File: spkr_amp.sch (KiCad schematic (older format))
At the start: 4 parts, among them U2 FSA2275UMX, U3 TPA2006D1DRBR

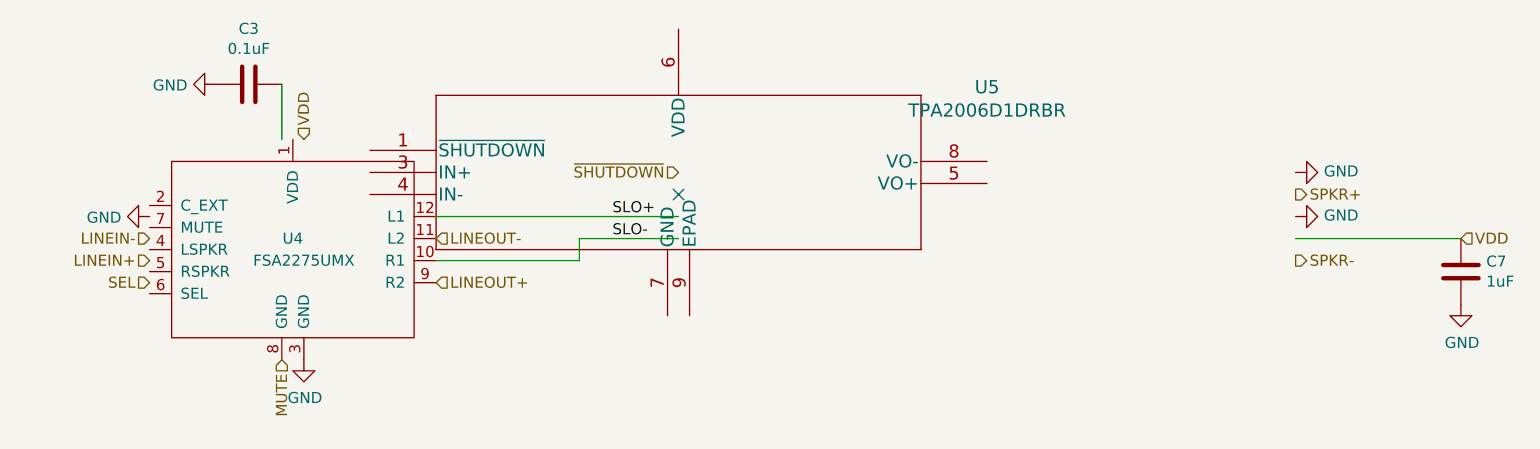
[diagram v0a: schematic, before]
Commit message: Lots of schematic cleanup and board tweaking
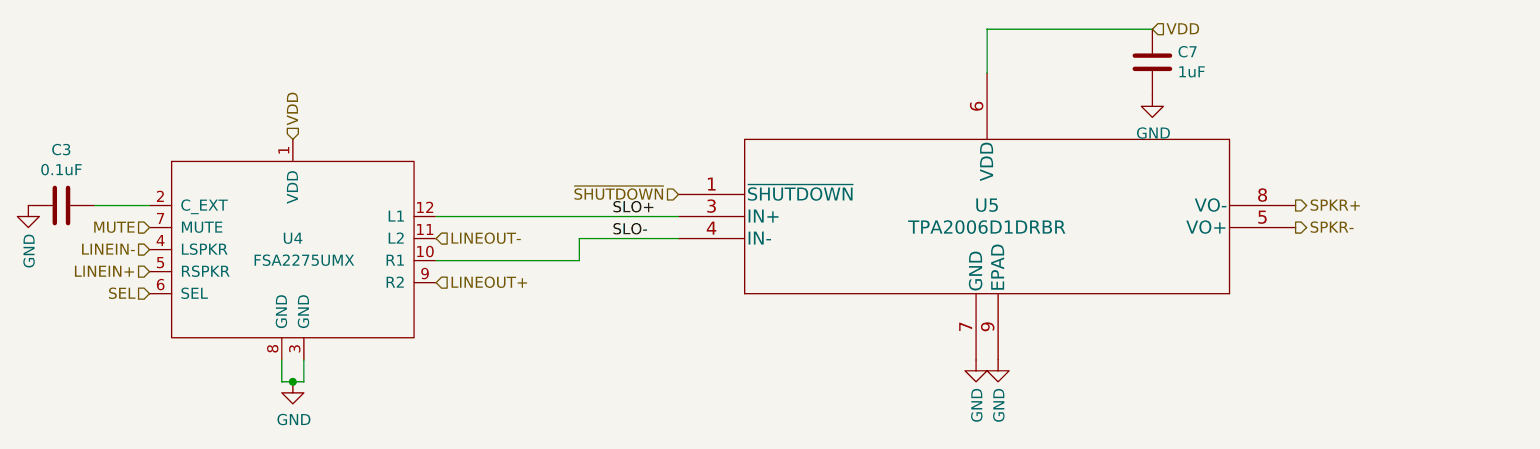
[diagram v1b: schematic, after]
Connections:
- wire segments 6 -> 11
- no-connect marks 1 -> 0
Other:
- moved on the sheet: C3, C7, U5
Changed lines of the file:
@@
 $Descr A4 11693 8268
 encoding utf-8
-Sheet 3 3
+Sheet 2 3
 Title ""
 Date ""
@@
 L TPA2006D1DRBR:TPA2006D1DRBR U?
 U 1 1 6026AF34
-P 5500 3300
+P 6900 3500
 AR Path="/6026AF34" Ref="U?"  Part="1"
 AR Path="/6026A3BE/6026AF34" Ref="U3"  Part="1"
 AR Path="/60276BEA/6026AF34" Ref="U5"  Part="1"
-F 0 "U5" H 6900 3687 60  0000 C CNN
-F 1 "TPA2006D1DRBR" H 6900 3581 60  0000 C CNN
-F 2 "footprints:TPA2006D1DRBR" H 6900 3540 60  0001 C CNN
-F 3 "" H 5500 3300 60  0000 C CNN
-	1    5500 3300
+F 0 "U5" H 6900 3550 60  0000 C CNN
+F 1 "TPA2006D1DRBR" H 6900 3450 60  0000 C CNN
+F 2 "footprints:TPA2006D1DRBR" H 8300 3740 60  0001 C CNN
+F 3 "" H 6900 3500 60  0000 C CNN
+	1    6900 3500
 	1    0    0    -1
 $EndComp
@@
 L power:GND #PWR06
 U 1 1 6027011E
-P 8300 3300
+P 6950 4150
 AR Path="/6026A3BE/6027011E" Ref="#PWR06"  Part="1"
 AR Path="/60276BEA/6027011E" Ref="#PWR011"  Part="1"
-F 0 "#PWR011" H 8300 3050 50  0001 C CNN
-F 1 "GND" V 8305 3172 50  0000 R CNN
-F 2 "" H 8300 3300 50  0001 C CNN
-F 3 "" H 8300 3300 50  0001 C CNN
-	1    8300 3300
-	0    -1   -1   0
+F 0 "#PWR011" H 6950 3900 50  0001 C CNN
+F 1 "GND" V 6955 4022 50  0000 R CNN
+F 2 "" H 6950 4150 50  0001 C CNN
+F 3 "" H 6950 4150 50  0001 C CNN
+	1    6950 4150
+	1    0    0    -1
 $EndComp
 $Comp
 L power:GND #PWR07
 U 1 1 60270A57
-P 8300 3500
+P 6850 4150
 AR Path="/6026A3BE/60270A57" Ref="#PWR07"  Part="1"
 AR Path="/60276BEA/60270A57" Ref="#PWR012"  Part="1"
-F 0 "#PWR012" H 8300 3250 50  0001 C CNN
-F 1 "GND" V 8305 3372 50  0000 R CNN
-F 2 "" H 8300 3500 50  0001 C CNN
-F 3 "" H 8300 3500 50  0001 C CNN
-	1    8300 3500
-	0    -1   -1   0
-$EndComp
-NoConn ~ 5500 3400
-Text HLabel 9050 3600 2    50   Input ~ 0
-VDD
-Text HLabel 8300 3400 2    50   Output ~ 0
-SPKR+
-Text HLabel 8300 3700 2    50   Output ~ 0
-SPKR-
-Text HLabel 3800 3150 1    50   Input ~ 0
-VDD
-$Comp
-L power:GND #PWR05
-U 1 1 6027124D
-P 3800 4150
-AR Path="/6026A3BE/6027124D" Ref="#PWR05"  Part="1"
-AR Path="/60276BEA/6027124D" Ref="#PWR010"  Part="1"
-F 0 "#PWR010" H 3800 3900 50  0001 C CNN
-F 1 "GND" H 3805 3977 50  0000 C CNN
-F 2 "" H 3800 4150 50  0001 C CNN
-F 3 "" H 3800 4150 50  0001 C CNN
-	1    3800 4150
+F 0 "#PWR012" H 6850 3900 50  0001 C CNN
+F 1 "GND" V 6855 4022 50  0000 R CNN
+F 2 "" H 6850 4150 50  0001 C CNN
+F 3 "" H 6850 4150 50  0001 C CNN
+	1    6850 4150
 	1    0    0    -1
 $EndComp
-$Comp
-L power:GND #PWR03
-U 1 1 6027187C
-P 3100 3500
-AR Path="/6026A3BE/6027187C" Ref="#PWR03"  Part="1"
-AR Path="/60276BEA/6027187C" Ref="#PWR08"  Part="1"
-F 0 "#PWR08" H 3100 3250 50  0001 C CNN
-F 1 "GND" V 3105 3372 50  0000 R CNN
-F 2 "" H 3100 3500 50  0001 C CNN
-F 3 "" H 3100 3500 50  0001 C CNN
-	1    3100 3500
-	0    1    1    0
-$EndComp
-Text HLabel 5500 3300 0    50   Input ~ 0
+Text HLabel 7650 2650 2    50   Input ~ 0
+VDD
+Text HLabel 8300 3450 2    50   Output ~ 0
+SPKR+
+Text HLabel 8300 3550 2    50   Output ~ 0
+SPKR-
+Text HLabel 3750 3150 1    50   Input ~ 0
+VDD
+Text HLabel 5500 3400 0    50   Input ~ 0
 ~SHUTDOWN
-Text HLabel 3100 3700 0    50   Input ~ 0
+Text HLabel 3100 3750 0    50   Input ~ 0
 LINEIN+
-Text HLabel 3100 3600 0    50   Input ~ 0
+Text HLabel 3100 3650 0    50   Input ~ 0
 LINEIN-
-Text HLabel 3100 3800 0    50   Input ~ 0
+Text HLabel 3100 3850 0    50   Input ~ 0
 SEL
 Text HLabel 4400 3800 2    50   Input ~ 0
@@
 Text HLabel 4400 3600 2    50   Input ~ 0
 LINEOUT-
-Text HLabel 3700 4150 3    50   Input ~ 0
+Text HLabel 3100 3550 0    50   Input ~ 0
 MUTE
 $Comp
 L Device:C C2
 U 1 1 60273CC0
-P 3550 2900
+P 2700 3450
 AR Path="/6026A3BE/60273CC0" Ref="C2"  Part="1"
 AR Path="/60276BEA/60273CC0" Ref="C3"  Part="1"
-F 0 "C3" V 3298 2900 50  0000 C CNN
-F 1 "0.1uF" V 3389 2900 50  0000 C CNN
-F 2 "Capacitor_SMD:C_0402_1005Metric" H 3588 2750 50  0001 C CNN
-F 3 "~" H 3550 2900 50  0001 C CNN
-	1    3550 2900
+F 0 "C3" V 2448 3450 50  0000 C CNN
+F 1 "0.1uF" V 2539 3450 50  0000 C CNN
+F 2 "Capacitor_SMD:C_0402_1005Metric" H 2738 3300 50  0001 C CNN
+F 3 "~" H 2700 3450 50  0001 C CNN
+	1    2700 3450
 	0    1    1    0
 $EndComp
-Wire Wire Line
-	3700 2900 3700 3150
 $Comp
 L power:GND #PWR04
 U 1 1 60274CA1
-P 3400 2900
+P 2550 3450
 AR Path="/6026A3BE/60274CA1" Ref="#PWR04"  Part="1"
 AR Path="/60276BEA/60274CA1" Ref="#PWR09"  Part="1"
-F 0 "#PWR09" H 3400 2650 50  0001 C CNN
-F 1 "GND" V 3405 2772 50  0000 R CNN
-F 2 "" H 3400 2900 50  0001 C CNN
-F 3 "" H 3400 2900 50  0001 C CNN
-	1    3400 2900
-	0    1    1    0
+F 0 "#PWR09" H 2550 3200 50  0001 C CNN
+F 1 "GND" V 2555 3322 50  0000 R CNN
+F 2 "" H 2550 3450 50  0001 C CNN
+F 3 "" H 2550 3450 50  0001 C CNN
+	1    2550 3450
+	1    0    0    -1
 $EndComp
 Text Label 5200 3500 0    50   ~ 0
@@
 L Device:C C7
 U 1 1 6034D245
-P 9050 3750
+P 7650 2800
 AR Path="/60276BEA/6034D245" Ref="C7"  Part="1"
 AR Path="/6026A3BE/6034D245" Ref="C6"  Part="1"
-F 0 "C7" H 9165 3796 50  0000 L CNN
-F 1 "1uF" H 9165 3705 50  0000 L CNN
-F 2 "Capacitor_SMD:C_0402_1005Metric" H 9088 3600 50  0001 C CNN
-F 3 "~" H 9050 3750 50  0001 C CNN
-	1    9050 3750
+F 0 "C7" H 7765 2846 50  0000 L CNN
+F 1 "1uF" H 7765 2755 50  0000 L CNN
+F 2 "Capacitor_SMD:C_0402_1005Metric" H 7688 2650 50  0001 C CNN
+F 3 "~" H 7650 2800 50  0001 C CNN
+	1    7650 2800
 	1    0    0    -1
 $EndComp
 Wire Wire Line
-	8300 3600 9050 3600
+	6900 2650 7650 2650
 $Comp
 L power:GND #PWR0105
 U 1 1 6034E328
-P 9050 3900
+P 7650 2950
 AR Path="/60276BEA/6034E328" Ref="#PWR0105"  Part="1"
 AR Path="/6026A3BE/6034E328" Ref="#PWR0104"  Part="1"
-F 0 "#PWR0105" H 9050 3650 50  0001 C CNN
-F 1 "GND" H 9055 3727 50  0000 C CNN
-F 2 "" H 9050 3900 50  0001 C CNN
-F 3 "" H 9050 3900 50  0001 C CNN
-	1    9050 3900
+F 0 "#PWR0105" H 7650 2700 50  0001 C CNN
+F 1 "GND" H 7655 2777 50  0000 C CNN
+F 2 "" H 7650 2950 50  0001 C CNN
+F 3 "" H 7650 2950 50  0001 C CNN
+	1    7650 2950
 	1    0    0    -1
 $EndComp
+Wire Wire Line
+	6900 2650 6900 2850
+$Comp
+L power:GND #PWR0107
+U 1 1 6043B2A1
+P 3750 4250
+AR Path="/6026A3BE/6043B2A1" Ref="#PWR0107"  Part="1"
+AR Path="/60276BEA/6043B2A1" Ref="#PWR0108"  Part="1"
+F 0 "#PWR0108" H 3750 4000 50  0001 C CNN
+F 1 "GND" H 3755 4077 50  0000 C CNN
+F 2 "" H 3750 4250 50  0001 C CNN
+F 3 "" H 3750 4250 50  0001 C CNN
+	1    3750 4250
+	1    0    0    -1
+$EndComp
+Wire Wire Line
+	3800 4150 3800 4250
+Wire Wire Line
+	3800 4250 3750 4250
+Wire Wire Line
+	3700 4250 3700 4150
+Connection ~ 3750 4250
+Wire Wire Line
+	3750 4250 3700 4250
+Wire Wire Line
+	2850 3450 3100 3450
 $EndSCHEMATC
